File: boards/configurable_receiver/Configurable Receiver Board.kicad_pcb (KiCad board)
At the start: 4 copper layers, 38.9 x 29.3 mm, 21 parts, among them J4 NeoPixel, P4 SERIAL, SW1 Switch_SPDT_x2, SW2 Switch_DPST, SW3 SW_DIP_x04, U0 10118194, U1 LM3671, U3 ESP-12F, U7 SN74LVC1T45

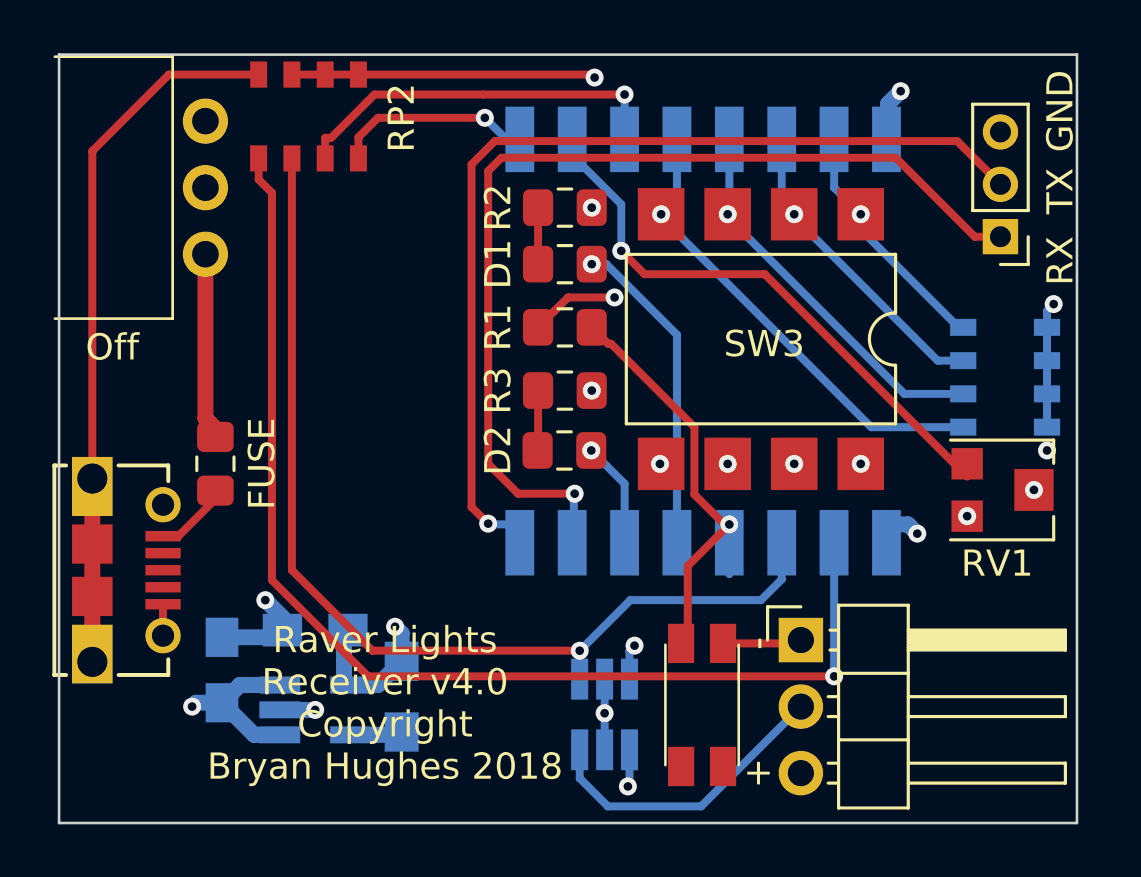
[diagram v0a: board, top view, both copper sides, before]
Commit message: Finished v4.5 of the receiver board
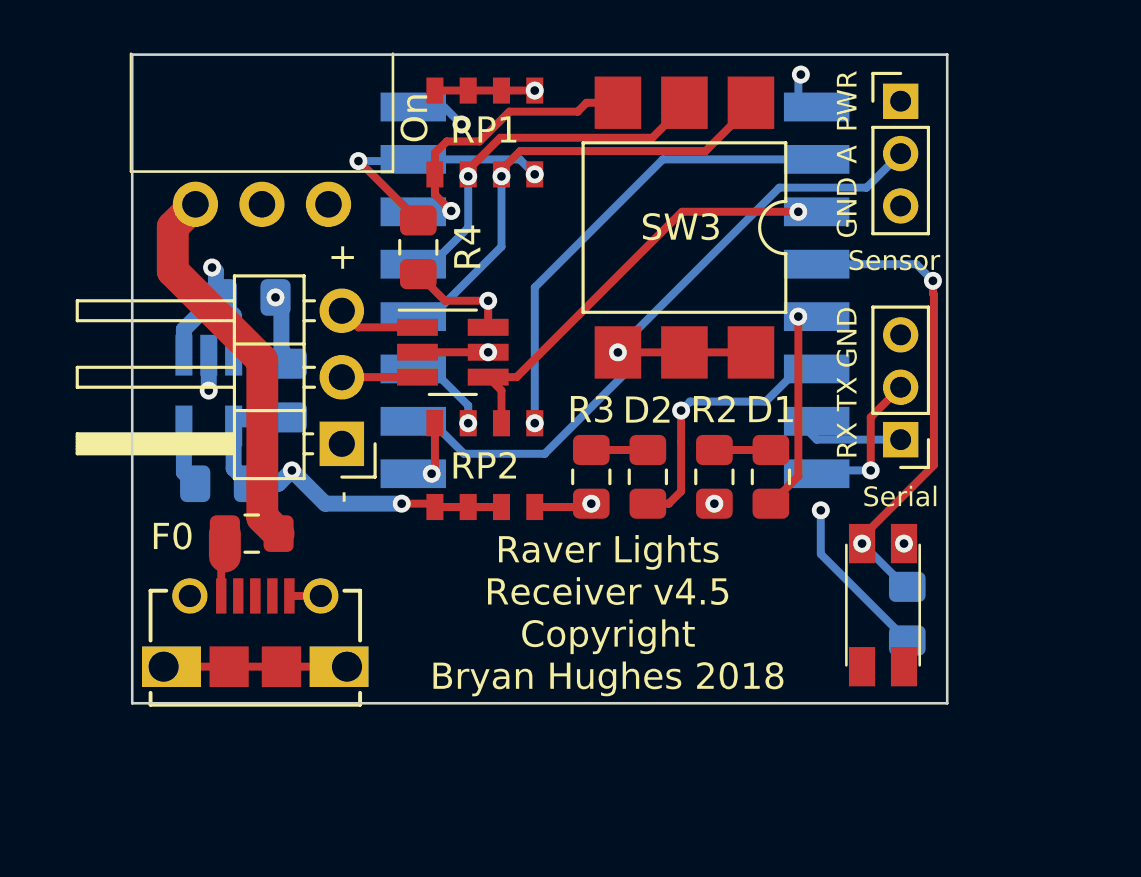
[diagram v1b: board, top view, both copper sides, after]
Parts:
- removed RV1: R_POT, nebrius-switch:TC33-potentiometer
- added P1: SENSOR, Connector_PinHeader_2.00mm:PinHeader_1x03_P2.00mm_Vertical, F.Cu at (126.1, 104.9)
- added R4: 0, Resistor_SMD:R_0805_2012Metric_Pad1.15x1.40mm_HandSolder, F.Cu at (107.6, 110.5)
- C1, C2: footprint Capacitors_SMD:C_0805_HandSoldering -> Capacitor_SMD:C_0805_2012Metric_Pad1.15x1.40mm_HandSolder
- L1: footprint Resistors_SMD:R_0805_HandSoldering -> Resistor_SMD:R_0805_2012Metric_Pad1.15x1.40mm_HandSolder
- P4: footprint Pin_Headers:Pin_Header_Straight_1x03_Pitch2.00mm -> Connector_PinHeader_2.00mm:PinHeader_1x03_P2.00mm_Vertical
- R1: moved to B.Cu
- RP1, U7: moved to F.Cu
- SW3: value SW_DIP_x04 -> SW_DIP_x03; footprint Package_DIP:SMDIP-8_W9.53mm -> Package_DIP:SMDIP-6_W9.53mm
- moved RP1 22.0 mm to (110.2, 106.1), turned to 0 degrees
- moved J4 19.1 mm to (104.7, 118.0), turned to 180 degrees
- moved R1 17.0 mm to (126.3, 124.5), turned to 90 degrees
- moved U7 15.0 mm to (109.0, 114.5), turned to 0 degrees
- moved RP2 14.9 mm to (110.2, 118.8), turned to 180 degrees
- moved C1 14.3 mm to (101.2, 112.4), turned to 0 degrees
- moved U1 12.9 mm to (99.6, 116.0), turned to 270 degrees
- moved U3 12.5 mm to (108.1, 119.2), turned to 0 degrees
- moved R2 11.8 mm to (118.9, 119.3), turned to 270 degrees
- moved D1 11.3 mm to (121.1, 119.3), turned to 270 degrees
- moved L1 10.6 mm to (100.1, 119.5), turned to 0 degrees
- moved C2 9.20 mm to (102.7, 116.0), turned to 90 degrees
- moved P4 8.63 mm to (126.1, 117.9)
- moved SW2 7.89 mm to (125.4, 124.2)
- moved U0 7.23 mm to (101.4, 126.5), turned to 0 degrees
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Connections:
- RP1 pad 4: Net-(RP1-Pad4) -> Net-(R4-Pad2)
- SW3 pad 1: Net-(RP1-Pad4) -> Net-(RP1-Pad3)
- SW3 pad 2: Net-(RP1-Pad3) -> Net-(RP1-Pad2)
- SW3 pad 3: Net-(RP1-Pad2) -> Net-(RP1-Pad1)
- SW3 pad 4: Net-(RP1-Pad1) -> VCC
- U3 pad 4: Net-(RP1-Pad1) -> Net-(RP1-Pad3)
- U3 pad 6: Net-(RP1-Pad3) -> Net-(RP1-Pad1)
- U3 pad 7: Net-(RP1-Pad4) -> Net-(R4-Pad2)
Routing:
- net Net-(P4-Pad1): track 37.2 -> 4.20 mm, vias 1 -> 0
- net Net-(P4-Pad2): track 36.5 -> 6.46 mm
- net Net-(RP2-Pad1): track 45.1 -> 17.3 mm
- net Net-(RP2-Pad2): track 40.0 -> 16.4 mm
- net GND: track 44.7 -> 21.7 mm
- net Net-(RP2-Pad3): track 15.3 -> 2.65 mm
- net Net-(R4-Pad2): track 0.00 -> 10.2 mm, vias 0 -> 2
- net Net-(J4-Pad2): track 11.6 -> 2.89 mm
- net Net-(RP1-Pad4): track 8.62 -> 0.00 mm, vias 1 -> 0
- net Net-(F0-Pad1): track 6.81 -> 14.6 mm
- net VCC: track 25.6 -> 32.0 mm, vias 11 -> 6
- net Net-(RP1-Pad1): track 17.4 -> 11.0 mm
- net Net-(D2-Pad2): track 3.35 -> 9.68 mm
- net Net-(RP1-Pad3): track 11.2 -> 17.4 mm
- net Net-(RP2-Pad4): track 8.02 -> 1.98 mm
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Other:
- board size 38.9 x 29.3 mm -> 31.1 x 24.8 mm
- board text added: "A"
- board text added: "F0"
- board text added: "On"
- board text added: "PWR"
- board text added: "Raver Lights Receiver v4.5 Copyright Bryan Hughes 2018"
- board text added: "Sensor"
- board text added: "Serial"
- board text removed: "FUSE"
- board text removed: "Off"
- board text removed: "Raver Lights Receiver v4.0 Copyright Bryan Hughes 2018"
